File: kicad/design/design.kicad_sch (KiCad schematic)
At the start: 46 parts, among them J1 Conn_01x12_Pin, SW1 Switch, SW10 Switch, SW11 Switch, SW12 Switch, SW13 Switch, SW14 Switch, SW15 Switch, SW16 Switch, SW17 Switch, SW18 Switch, SW19 Switch, SW2 Switch, SW20 Switch, SW21 Switch, SW22 Switch, SW3 Switch, SW4 Switch, SW5 Switch, SW6 Switch, SW7 Switch, SW8 Switch, SW9 Switch, U1 Raspberry_Pi_Pico

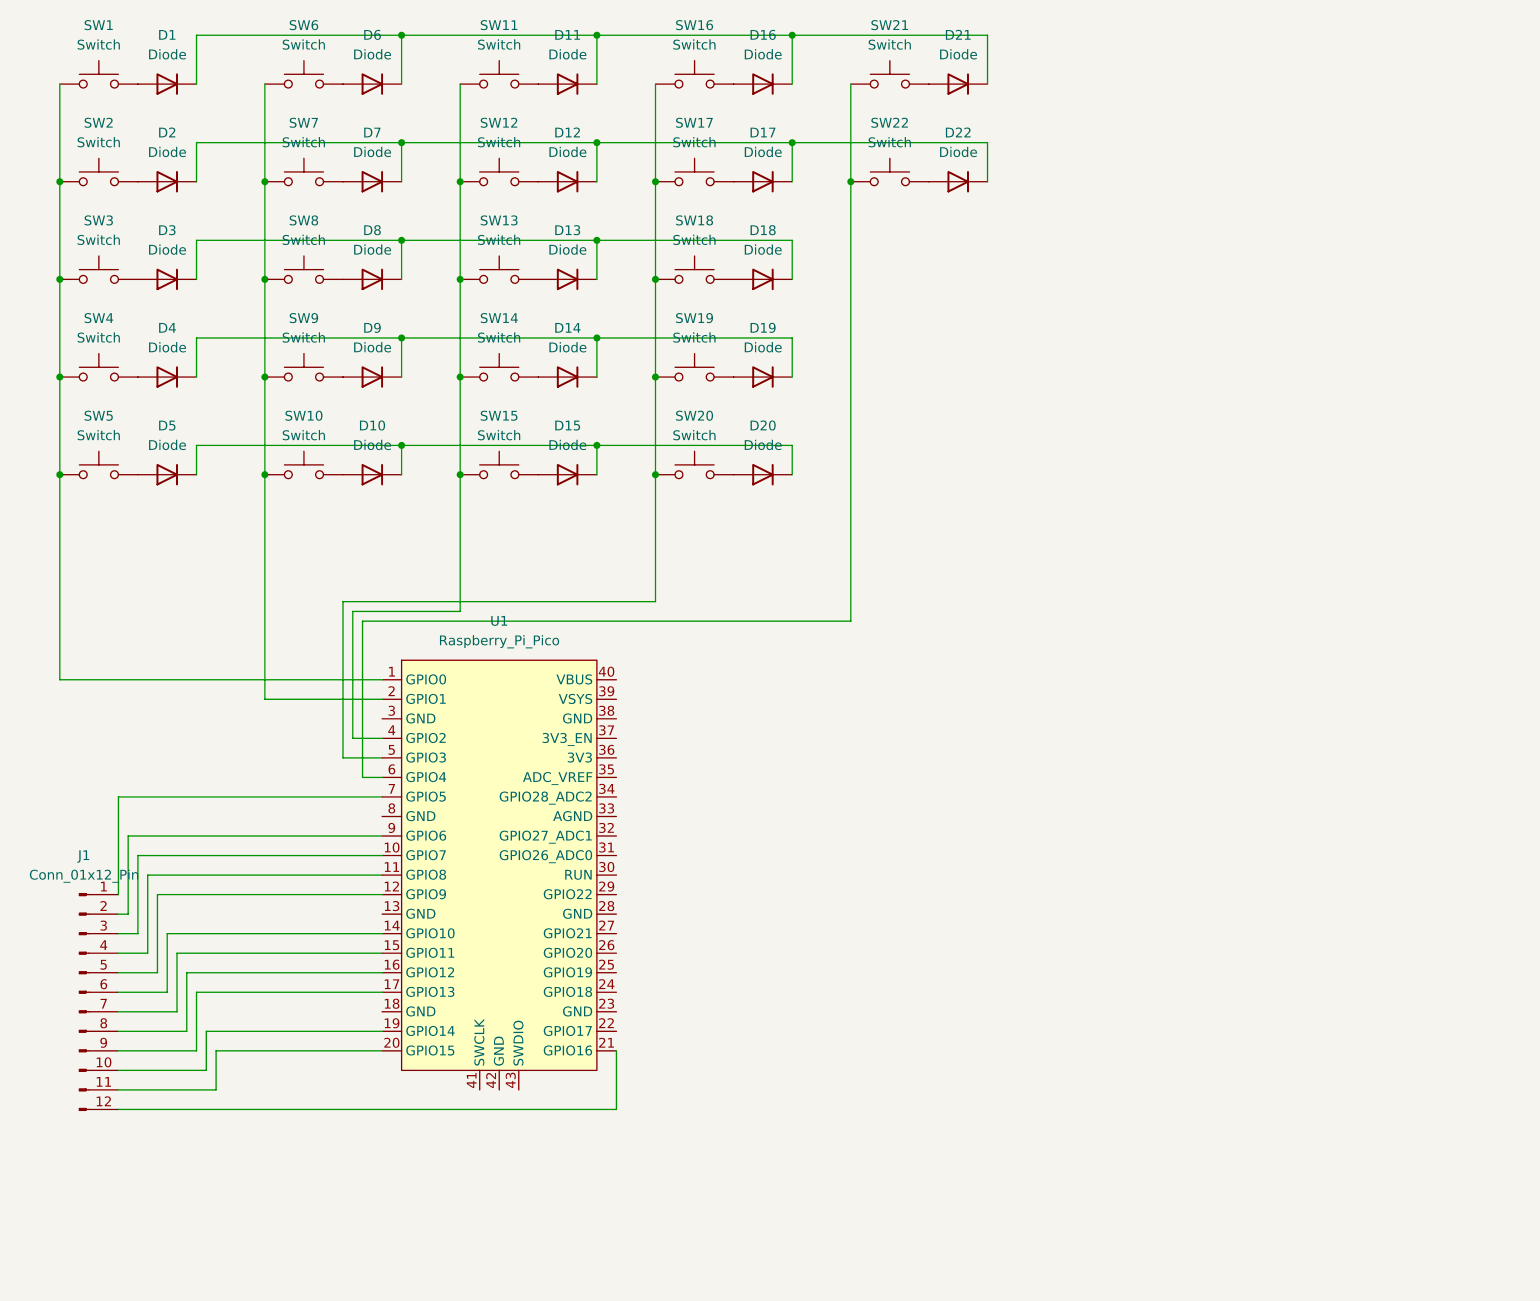
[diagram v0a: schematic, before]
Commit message: PCB Components Placed
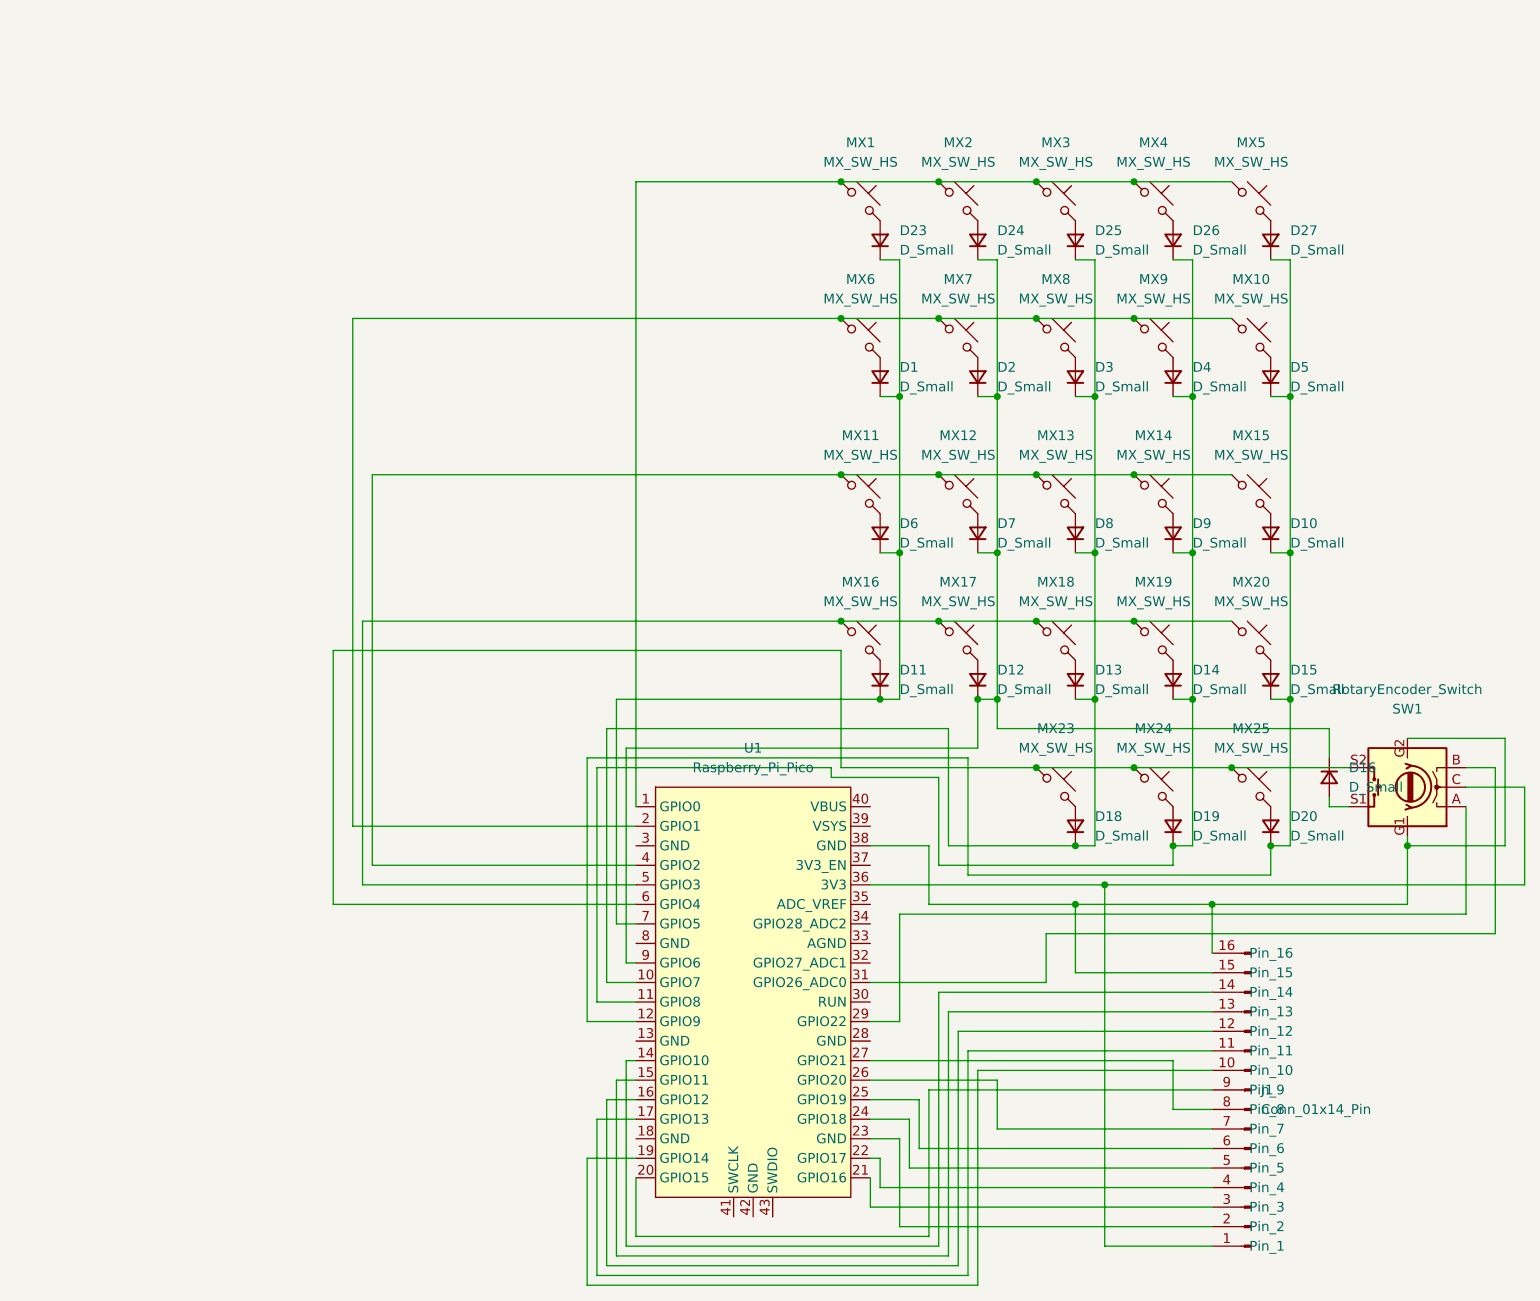
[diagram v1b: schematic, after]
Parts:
- removed D1, D10, D11, D12, D13, D14, D15, D16, D17, D18, D19, D2, D20, D21, D22, D3, D4, D5, D6, D7, D8, D9: Diode, symbol ScottoKeebs:Placeholder_Diode
- removed J1: Conn_01x12_Pin, symbol Connector:Conn_01x12_Pin
- removed SW1, SW10, SW11, SW12, SW13, SW14, SW15, SW16, SW17, SW18, SW19, SW2, SW20, SW21, SW22, SW3, SW4, SW5, SW6, SW7, SW8, SW9: Switch, symbol ScottoKeebs:Placeholder_Switch
- added D1, D10, D11, D12, D13, D14, D15, D16, D18, D19, D2, D20, D23, D24, D25, D26, D27, D3, D4, D5, D6, D7, D8, D9: D_Small, Diode_SMD:D_SOD-123, symbol Device:D_Small
- added J1: Conn_01x14_Pin, CustomKicad:XF3M-1415-1B, symbol Connector:Conn_01x16_Pin
- added MX1, MX10, MX11, MX12, MX13, MX14, MX15, MX16, MX17, MX18, MX19, MX2, MX20, MX23, MX24, MX25, MX3, MX4, MX5, MX6, MX7, MX8, MX9: MX_SW_HS, PCM_marbastlib-mx:SW_MX_HS_1u, symbol PCM_marbastlib-mx:MX_SW_HS
- added SW1: RotaryEncoder_Switch, CustomKicad:PEC12R-42, symbol Device:RotaryEncoder_Switch
- U1: footprint ScottoKeebs_MCU:Raspberry_Pi_Pico -> CustomKicad:RPi_Pico_SMD_TH
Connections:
- net at U1.4 (GPIO2): now also MX11.1, MX12.1, MX13.1, MX14.1, MX15.1
- net at U1.1 (GPIO0): now also MX1.1, MX2.1, MX3.1, MX4.1, MX5.1
- net at U1.6 (GPIO4): now also MX23.1, MX24.1, MX25.1, SW1.S2
- net at U1.2 (GPIO1): now also MX10.1, MX6.1, MX7.1, MX8.1, MX9.1
- net at U1.7 (GPIO5): now also D1.1 (K), D11.1 (K), D23.1 (K), D6.1 (K)
- net at U1.19 (GPIO14): now also J1.10 (Pin_10)
- net at U1.20 (GPIO15): now also J1.9 (Pin_9)
- net at U1.21 (GPIO16): now also J1.3 (Pin_3)
- net at U1.9 (GPIO6): now also D12.1 (K), D16.1 (K), D2.1 (K), D24.1 (K), D7.1 (K)
- net at U1.10 (GPIO7): now also D13.1 (K), D18.1 (K), D25.1 (K), D3.1 (K), D8.1 (K)
- net at U1.11 (GPIO8): now also D14.1 (K), D19.1 (K), D26.1 (K), D4.1 (K), D9.1 (K)
- net at U1.12 (GPIO9): now also D10.1 (K), D15.1 (K), D20.1 (K), D27.1 (K), D5.1 (K)
- net at U1.14 (GPIO10): now also J1.14 (Pin_14)
- net at U1.15 (GPIO11): now also J1.13 (Pin_13)
- net at U1.16 (GPIO12): now also J1.12 (Pin_12)
- net at U1.17 (GPIO13): now also J1.11 (Pin_11)
- net at U1.5 (GPIO3): now also MX16.1, MX17.1, MX18.1, MX19.1, MX20.1
- net at U1.22 (GPIO17): now also J1.4 (Pin_4)
- net at U1.23 (GND): now also J1.2 (Pin_2)
- net at U1.24 (GPIO18): now also J1.5 (Pin_5)
- net at U1.25 (GPIO19): now also J1.6 (Pin_6)
- net at U1.26 (GPIO20): now also J1.7 (Pin_7)
- net at U1.27 (GPIO21): now also J1.8 (Pin_8)
- net at U1.29 (GPIO22): now also SW1.A
- net at U1.31 (GPIO26_ADC0): now also SW1.B
- net at U1.36 (3V3): now also J1.1 (Pin_1), SW1.C
- net at U1.38 (GND): now also J1.15 (Pin_15), J1.16 (Pin_16), SW1.G1, SW1.G2
- new net: D8.2 (A), MX13.2
- new net: D15.2 (A), MX20.2
- new net: D1.2 (A), MX6.2
- new net: D5.2 (A), MX10.2
- new net: D2.2 (A), MX7.2
- new net: D24.2 (A), MX2.2
- new net: D14.2 (A), MX19.2
- new net: D27.2 (A), MX5.2
- new net: D19.2 (A), MX24.2
- new net: D10.2 (A), MX15.2
- new net: D26.2 (A), MX4.2
- new net: D9.2 (A), MX14.2
- new net: D18.2 (A), MX23.2
- new net: D11.2 (A), MX16.2
- new net: D7.2 (A), MX12.2
- new net: D13.2 (A), MX18.2
- new net: D4.2 (A), MX9.2
- new net: D12.2 (A), MX17.2
- new net: D6.2 (A), MX11.2
- new net: D25.2 (A), MX3.2
- new net: D3.2 (A), MX8.2
- new net: D16.2 (A), SW1.S1
- new net: D20.2 (A), MX25.2
- new net: D23.2 (A), MX1.2
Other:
- moved on the sheet: U1
